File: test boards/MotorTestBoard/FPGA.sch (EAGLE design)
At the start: 2 parts, among them X1 87758-4016, X2 87758-4016

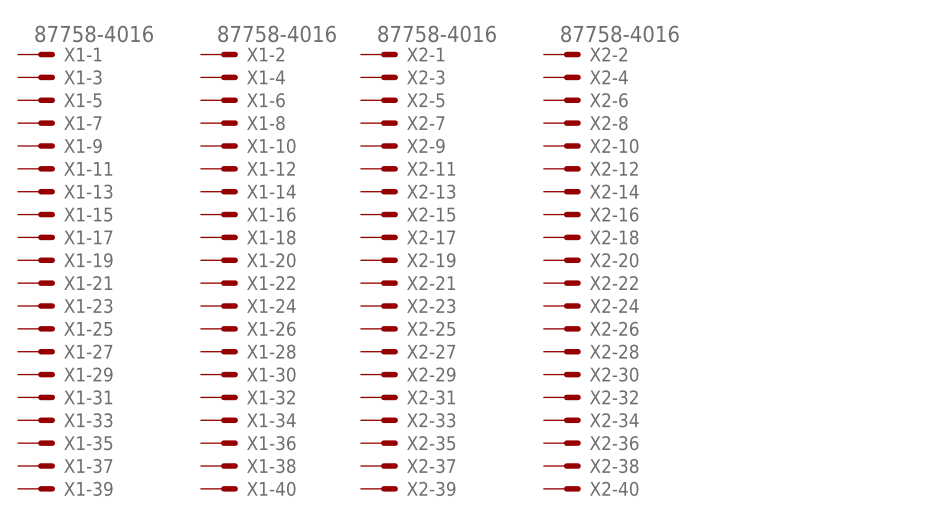
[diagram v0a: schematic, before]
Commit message: FPGA Labelling
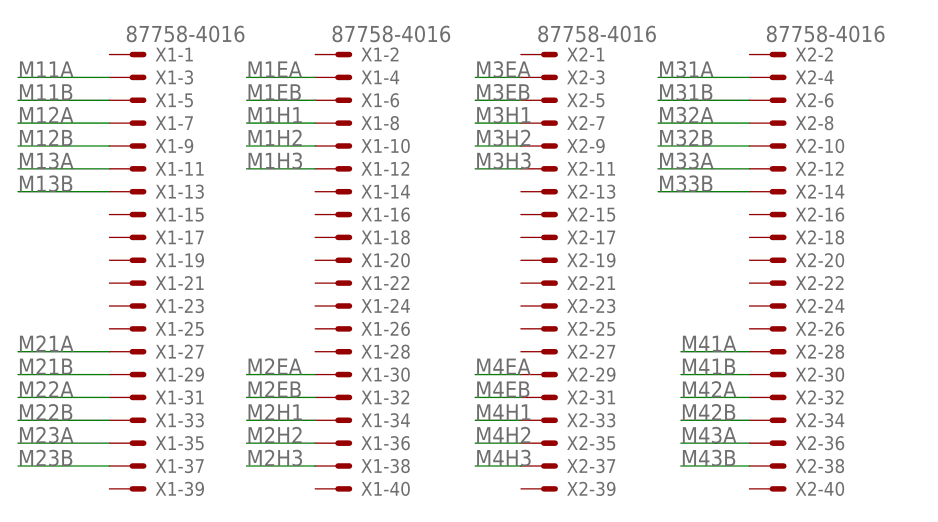
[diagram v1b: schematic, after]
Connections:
- new net M11A: X1-3.S
- new net M11B: X1-5.S
- new net M12A: X1-7.S
- new net M12B: X1-9.S
- new net M13A: X1-11.S
- new net M13B: X1-13.S
- new net M1EA: X1-4.S
- new net M1EB: X1-6.S
- new net M1H1: X1-8.S
- new net M1H2: X1-10.S
- new net M1H3: X1-12.S
- new net M21A: X1-27.S
- new net M21B: X1-29.S
- new net M22A: X1-31.S
- new net M22B: X1-33.S
- new net M23A: X1-35.S
- new net M23B: X1-37.S
- new net M2EA: X1-30.S
- new net M2EB: X1-32.S
- new net M2H1: X1-34.S
- new net M2H2: X1-36.S
- new net M2H3: X1-38.S
- new net M31A: X2-4.S
- new net M31B: X2-6.S
- new net M32A: X2-8.S
- new net M32B: X2-10.S
- new net M33A: X2-12.S
- new net M33B: X2-14.S
- new net M3EA: X2-3.S
- new net M3EB: X2-5.S
- new net M3H1: X2-7.S
- new net M3H2: X2-9.S
- new net M3H3: X2-11.S
- new net M41A: X2-28.S
- new net M41B: X2-30.S
- new net M42A: X2-32.S
- new net M42B: X2-34.S
- new net M43A: X2-36.S
- new net M43B: X2-38.S
- new net M4EA: X2-29.S
- new net M4EB: X2-31.S
- new net M4H1: X2-33.S
- new net M4H2: X2-35.S
- new net M4H3: X2-37.S
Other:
- moved on the sheet: X1-1, X1-10, X1-11, X1-12, X1-13, X1-14, X1-15, X1-16, X1-17, X1-18, X1-19, X1-2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
